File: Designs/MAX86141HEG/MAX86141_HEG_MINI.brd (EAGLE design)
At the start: 76 x 10 mm, 19 parts, among them U1 MAX86141ENP+T, U3 TXBN0304RUTR, U4 LP5907MFX-3.3/NOPB

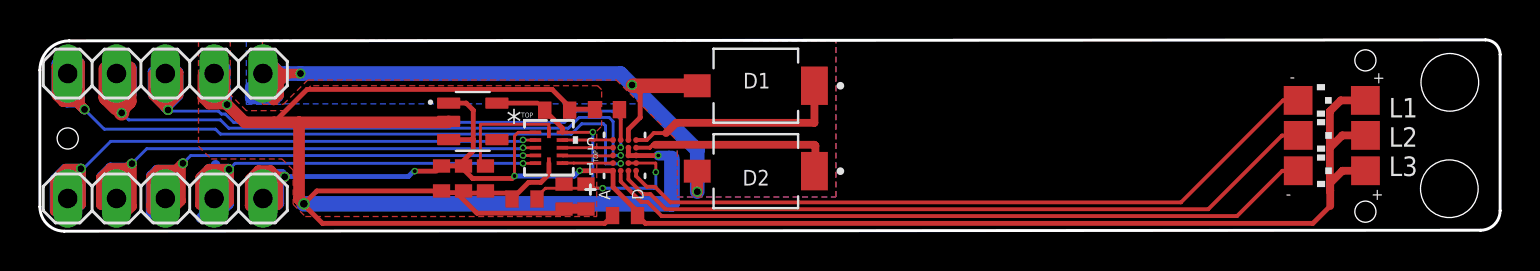
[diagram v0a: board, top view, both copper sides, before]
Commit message: quality improvements to design (hopefully)
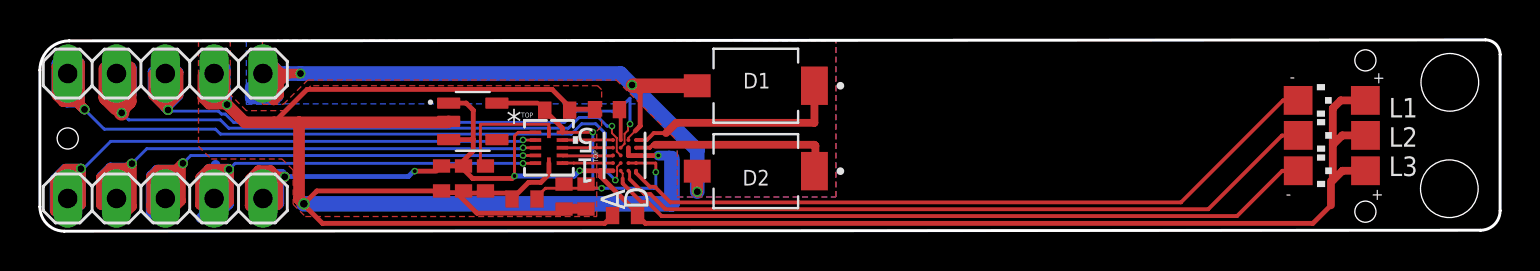
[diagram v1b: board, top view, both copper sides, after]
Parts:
- U1: device MAX86141:21-100134A_20 -> MAX86141:21-100134_N201A2-1_MXM
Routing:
- net GPIO2: track 39.8 -> 41.8 mm
- net INT: track 50.0 -> 51.0 mm
- net 3.3V: track 95.2 -> 94.5 mm

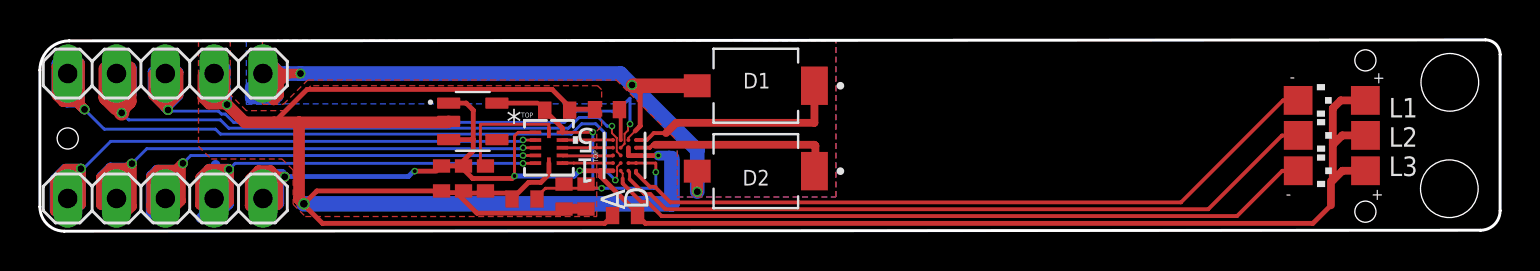
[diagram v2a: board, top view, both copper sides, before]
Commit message: reverted breakout board (trace spacing too narrow)
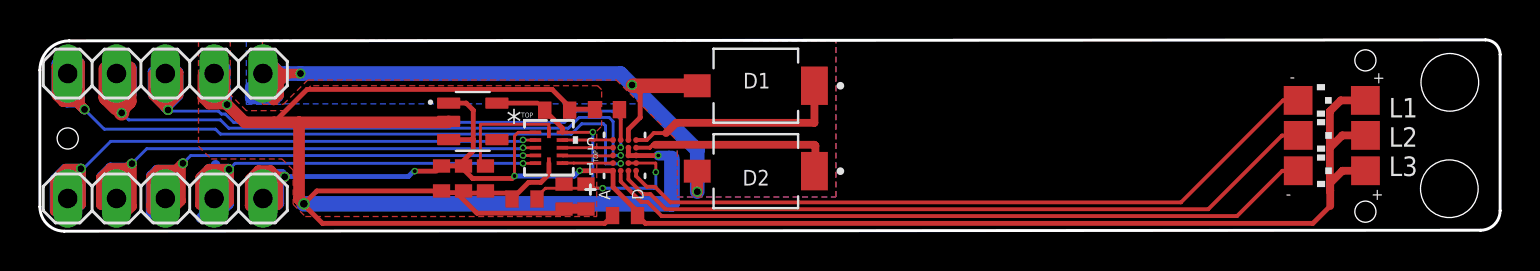
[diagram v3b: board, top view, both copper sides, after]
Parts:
- U1: device MAX86141:21-100134_N201A2-1_MXM -> MAX86141:21-100134A_20
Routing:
- net GPIO2: track 41.8 -> 39.8 mm
- net INT: track 51.0 -> 50.0 mm
- net 3.3V: track 94.5 -> 95.2 mm
